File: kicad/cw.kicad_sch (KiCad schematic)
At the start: 99 parts, among them J1 AUDIO, J2 KEY, Q1 NPN, Q10 NPN, Q11 NPN, Q2 NMOS, Q3 NPN, Q4 NPN, Q5 NPN, Q6 NPN, Q7 NPN, Q8 NPN, Q9 NPN, SW1 TX/RX, SW2 TX/RX, SW3 FREQ_SELECT, U1 Si5351A-B-GT, U3 PCF8574TS, U4 RC1602A

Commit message: Update cw.kicad_sch
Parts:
- removed L18, L23: L, symbol Device:L
- removed Q5: NPN, symbol Simulation_SPICE:NPN
- added C32, C33, C34, C36, C37, C38, C39, C40, C41: C, symbol Device:C
- added C35: 100n, symbol Device:C
- added R22: 1k, symbol Device:R
- added RV1, RV2, RV3, RV4: R_Potentiometer, symbol Device:R_Potentiometer
- added Y1, Y2, Y3, Y4, Y5, Y6, Y7, Y8: Crystal, symbol Device:Crystal
- C9: value C -> 100n
- R4, R5: value R -> 10k
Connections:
- net +12V: now also Q1.1 (C), R4.1; no longer C1.1, C9.1, L1.2
- net GND: now also C12.1, C32.1, C33.1, C37.1, C38.1, C39.1, R22.2; no longer Q1.3 (E), R4.2
- net at L7.2: now also C26.2; no longer C12.1
- net at C11.1, C20.2: now also C41.1; no longer C26.1
- net at Q1.2 (B), R5.1: now also C9.2, R4.2; no longer J2.T
- net at C15.2, C17.1: now also C26.1; no longer C16.1
- net at Q3.2 (B), R3.1: now also RV3.1; no longer C2.2, C31.2
- net at Q7.3 (E), R8.1: now also L1.1
- net at L19.1: now also C35.2; no longer C9.2
- new net: C16.1, L7.1
- new net: C35.1, Q1.3 (E), R22.1
- new net: C39.2, Y7.2, Y8.1
- new net: C40.1, Y8.2
- new net: C37.2, Y5.2, Y6.1
- new net: C38.2, Y6.2, Y7.1
- new net: C36.1, RV3.2
- new net: J2.T, RV1.1
- new net: C41.2, L1.2
- new net: C34.2, RV2.2
- new net: C29.1, C9.1, RV2.3
- new net: C36.2, Y5.1
- new net: C1.1, RV1.2
- new net: C1.2, Y1.1
- new net: C12.2, Y1.2, Y2.1
- new net: C32.2, Y2.2, Y3.1
- new net: C40.2, RV4.2
- new net: C33.2, Y3.2, Y4.1
- new net: C2.2, C31.2, RV4.3
- new net: C34.1, Y4.2
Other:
- moved on the sheet: AE1, C10, C11, C13, C14, C15, C16, C17, C2, C20, C21, C22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

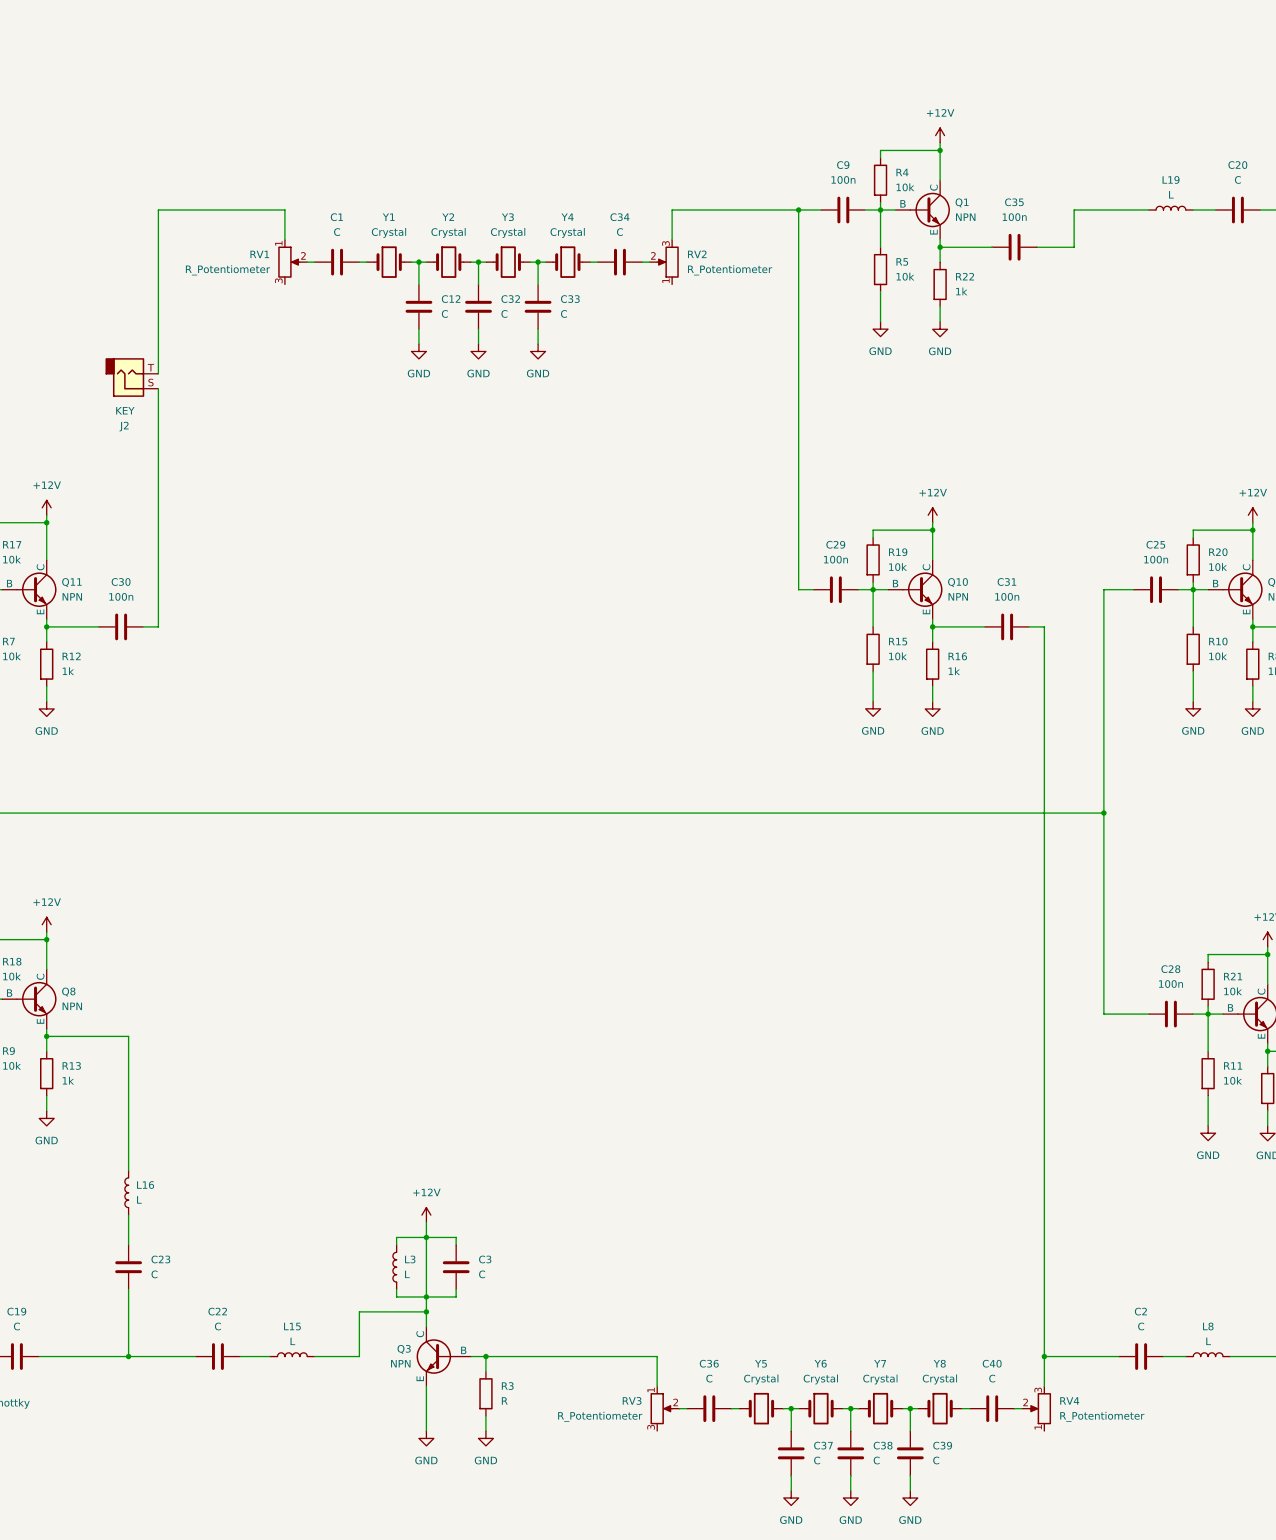
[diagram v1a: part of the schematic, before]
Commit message: Update cw.kicad_sch
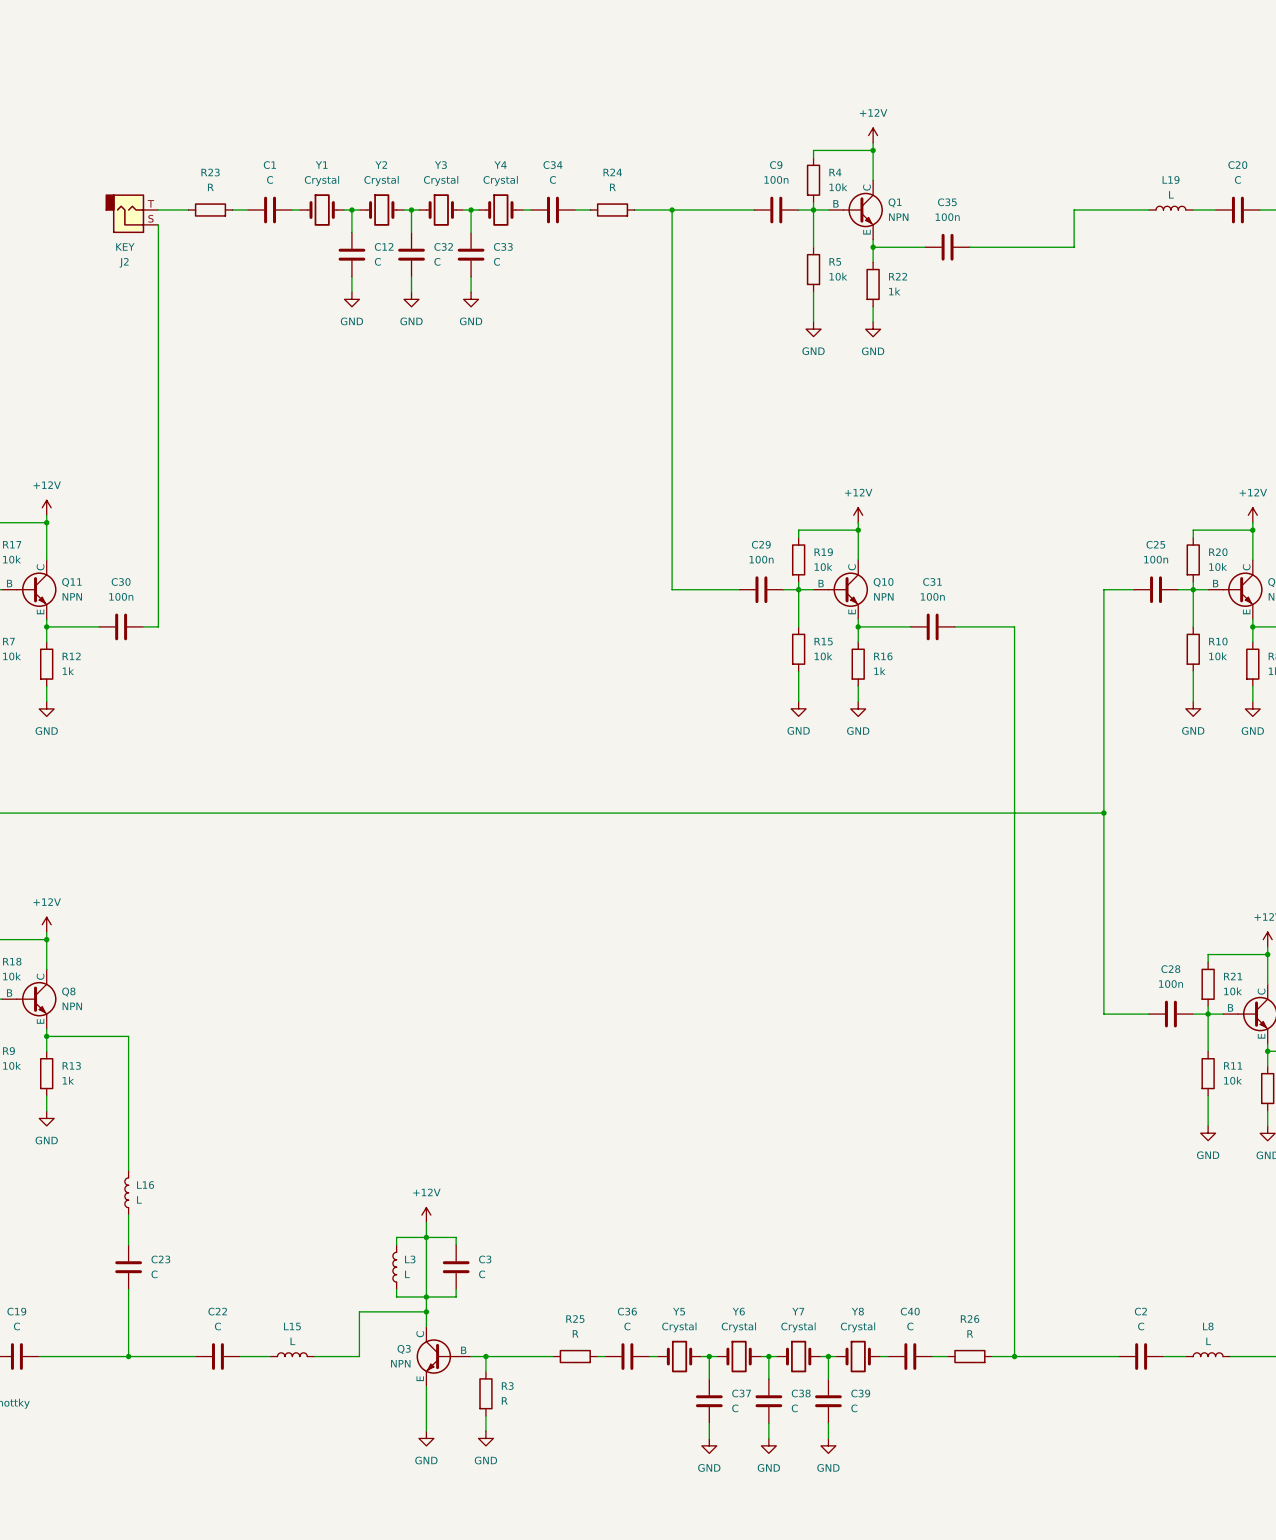
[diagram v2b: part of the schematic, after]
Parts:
- removed RV1, RV2, RV3, RV4: R_Potentiometer, symbol Device:R_Potentiometer
- added R23, R24, R25, R26: R, symbol Device:R
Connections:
- net at Q3.2 (B), R3.1: now also R25.1
- net at C36.1: now also R25.2
- net at J2.T: now also R23.1
- net at C34.2: now also R24.1
- net at C29.1, C9.1: now also R24.2
- net at C1.1: now also R23.2
- net at C40.2: now also R26.1
- net at C2.2, C31.2: now also R26.2
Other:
- moved on the sheet: C1, C12, C29, C31, C32, C33, C34, C35, C36, C37, C38, C39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
